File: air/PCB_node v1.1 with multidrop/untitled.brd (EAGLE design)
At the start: 150 x 100 mm, 121 parts, among them J1 10118193-0001LF, J2 10118193-0001LF, J3 U.FL-R-SMT(01), K1 351, K2 351, K3 SRD-05VDC-SL-C, K4 351, Q1 MMBT3904, Q10 S9013, Q11 PDTC114EU,115, Q2 MMBT3904, Q3 12MHz, Q4 S9013, Q5 S9013, Q6 S9013, Q7 12MHz, Q8 MMBT3904, Q9 MMBT3904, U1 CH340G, U10 ADS1115IDGSR, U11 PC817X2NIP0F, U12 NEO-M8N-0, U2 ESP32-WROOM-32D, U3 AMS1117, U4 PC817X2NIP0F, U5 PC817X2NIP0F, U6 PC817X2NIP0F, U7 CH340G, U8 AMS1117, U9 ESP32-WROOM-32D, X1 MSTBA2, X2 MSTBA2, X3 MSTBA4, X4 MSTBA3, X5 MSTBA2, X6 MSTBA4, X7 C-GRID-02-70543, X8 MSTBA2

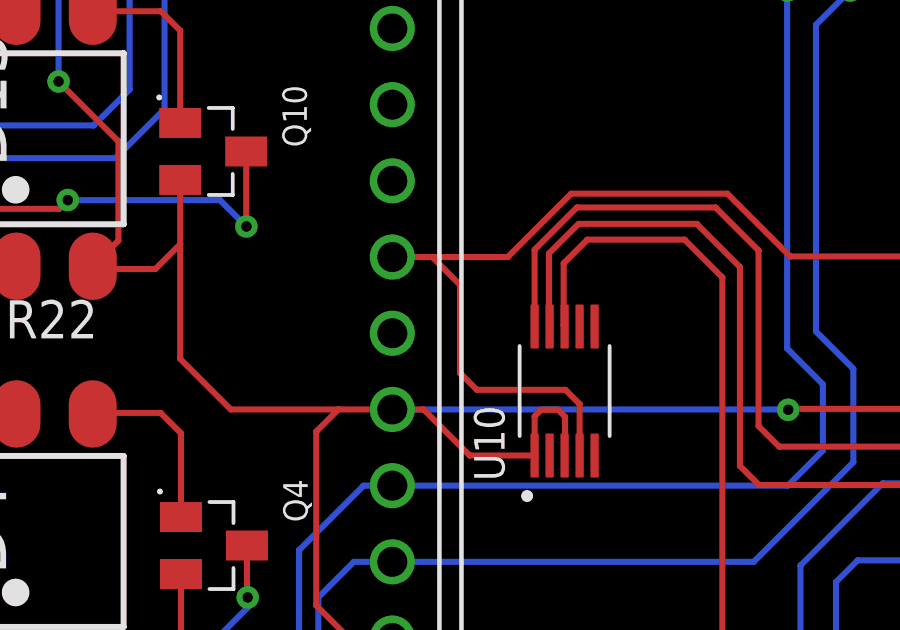
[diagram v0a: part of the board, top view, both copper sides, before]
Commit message: fix PCB
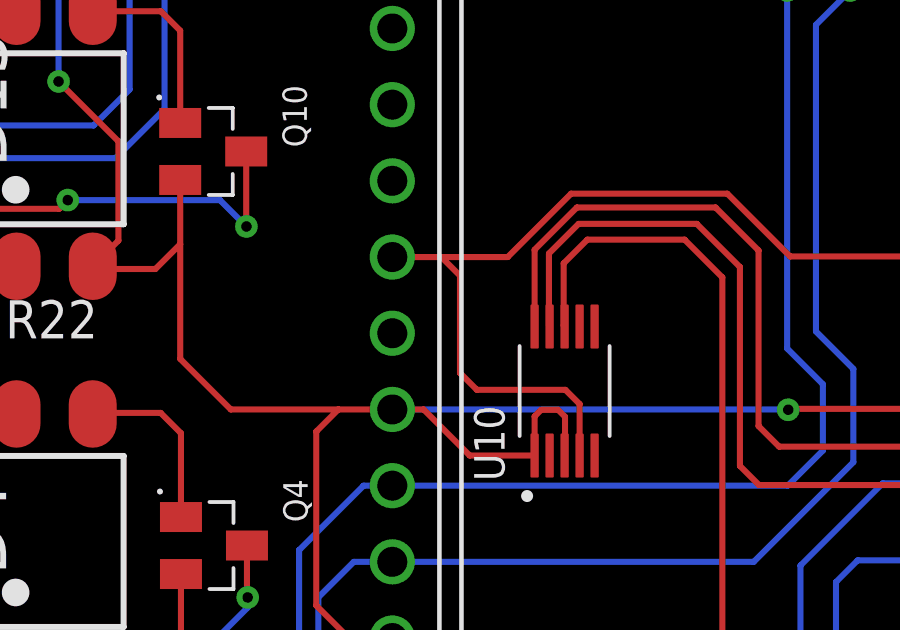
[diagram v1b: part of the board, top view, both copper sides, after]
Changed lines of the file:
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@@
 <wire x1="108.07954375" y1="30.049675" x2="105.128484375" y2="30.049675" width="0.2032" layer="1"/>
 <wire x1="105.128484375" y1="30.049675" x2="104.565653125" y2="30.61250625" width="0.2032" layer="1"/>
-<wire x1="104.565653125" y1="30.61250625" x2="104.565653125" y2="33.55030625" width="0.2032" layer="1"/>
-<wire x1="103.640440625" y1="34.47551875" x2="102.309053125" y2="34.47551875" width="0.2032" layer="1"/>
-<wire x1="104.565653125" y1="33.55030625" x2="103.640440625" y2="34.47551875" width="0.2032" layer="1"/>
+<wire x1="104.565653125" y1="30.61250625" x2="104.565653125" y2="33.85510625" width="0.2032" layer="1"/>
+<wire x1="103.945240625" y1="34.47551875" x2="102.309053125" y2="34.47551875" width="0.2032" layer="1"/>
+<wire x1="104.565653125" y1="33.85510625" x2="103.945240625" y2="34.47551875" width="0.2032" layer="1"/>
 <wire x1="120.04408125" y1="34.495728125" x2="115.568690625" y2="34.495728125" width="0.2032" layer="1"/>
 <wire x1="115.568690625" y1="34.495728125" x2="113.475909375" y2="36.588509375" width="0.2032" layer="1"/>
 <wire x1="113.475909375" y1="36.588509375" x2="108.2684125" y2="36.588509375" width="0.2032" layer="1"/>
-<wire x1="106.155421875" y1="34.47551875" x2="103.640440625" y2="34.47551875" width="0.2032" layer="1"/>
+<wire x1="106.155421875" y1="34.47551875" x2="103.945240625" y2="34.47551875" width="0.2032" layer="1"/>
 <wire x1="108.2684125" y1="36.588509375" x2="106.155421875" y2="34.47551875" width="0.2032" layer="1"/>
 <wire x1="136.611259375" y1="7.763196875" x2="132.775103125" y2="7.763196875" width="0.2032" layer="1"/>
